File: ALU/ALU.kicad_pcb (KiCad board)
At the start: 2 copper layers, 115 x 57 mm, 33 parts, among them J1 Conn_01x06_Pin, J2 Conn_01x08_Pin, J3 Conn_01x08_Pin, J4 Conn_01x10_Pin, U1 SN74F86N, U2 SN74F86N, U3 SN74HCT245N, U4 CD74HCT283E, U5 CD74HCT283E, U8 Dual D FF

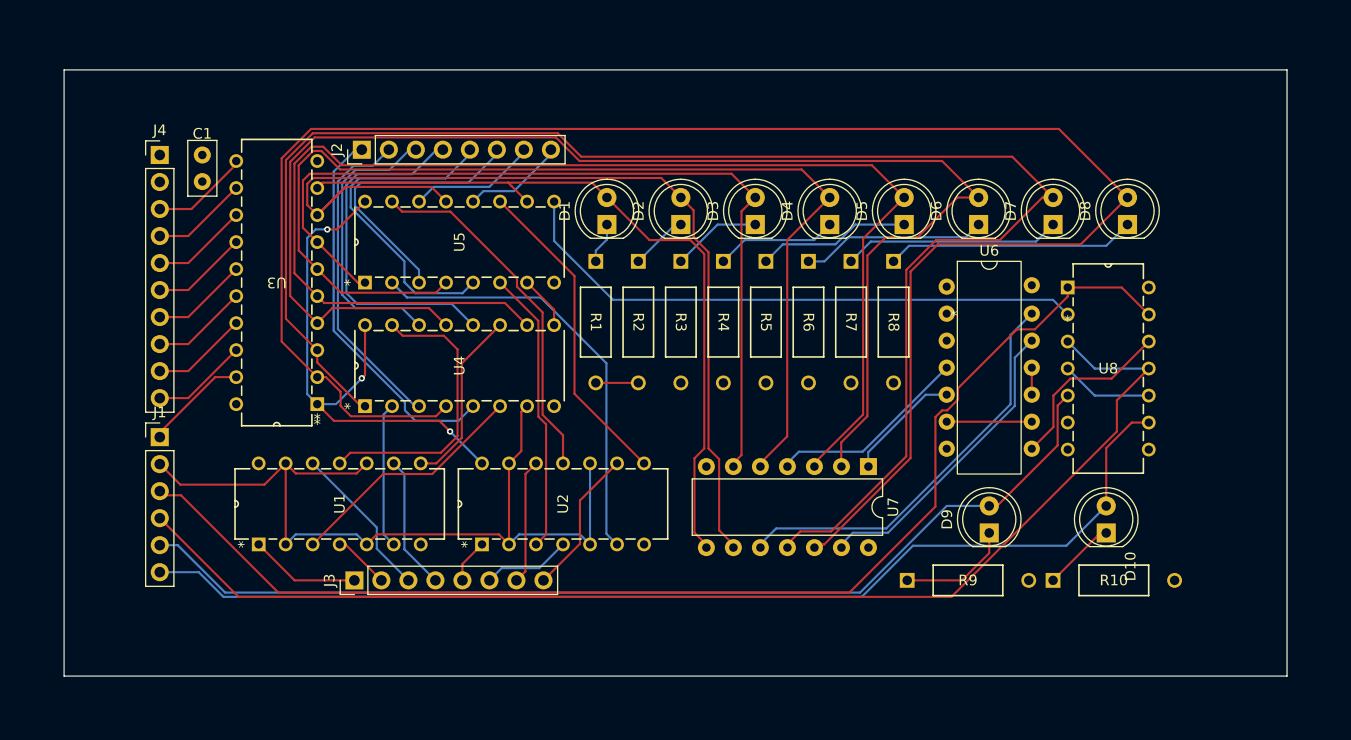
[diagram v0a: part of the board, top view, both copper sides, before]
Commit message: ALU layout complete
ALU layout complete
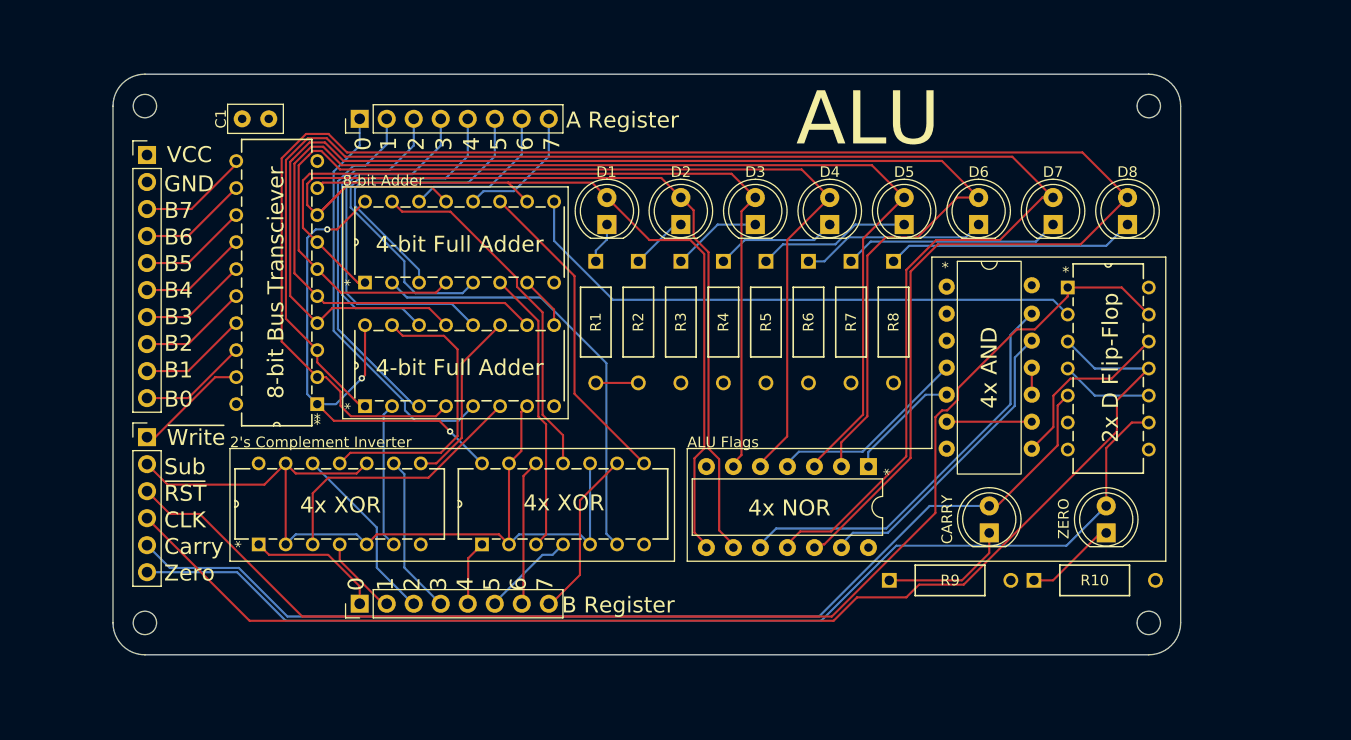
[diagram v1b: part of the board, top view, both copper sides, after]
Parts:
- added REF**: MountingHole_2.2mm_M2, MountingHole:MountingHole_2.2mm_M2, F.Cu at (78.6, 134.0)
- added REF**: MountingHole_2.2mm_M2, MountingHole:MountingHole_2.2mm_M2, F.Cu at (173.0, 134.0)
- added REF**: MountingHole_2.2mm_M2, MountingHole:MountingHole_2.2mm_M2, F.Cu at (78.6, 85.4)
- added REF**: MountingHole_2.2mm_M2, MountingHole:MountingHole_2.2mm_M2, F.Cu at (173.0, 85.4)
- moved C1 5.06 mm to (87.8, 86.6), turned to 0 degrees
- moved J2 2.91 mm to (98.8, 86.6)
- moved J3 2.26 mm to (98.8, 132.2)
- moved R10 1.80 mm to (162.2, 130.0)
- moved R9 1.69 mm to (148.6, 130.0)
- moved J1 1.20 mm to (78.8, 116.5)
- moved J4 1.20 mm to (78.8, 90.0)
- renumbered D9 to CARRY, D10 to ZERO
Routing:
- net /~{RST}: track 115.9 -> 119.4 mm
- net /CLK: track 115.3 -> 118.4 mm
- net /CARRY: track 97.1 -> 100.2 mm
- net /ZERO: track 103.9 -> 107.0 mm
- net /A6: track 12.0 -> 14.9 mm
- net /A7: track 9.59 -> 12.4 mm
- net /A5: track 26.5 -> 29.3 mm
- net /A4: track 31.3 -> 34.1 mm
- net /XOR0: track 23.0 -> 25.8 mm
- net /A3: track 33.8 -> 36.2 mm
- net /A2: track 27.1 -> 29.6 mm
- net /A0: track 36.1 -> 38.6 mm
- net /B2: track 14.7 -> 17.2 mm
- net /B3: track 12.6 -> 15.0 mm
- net /A1: track 30.5 -> 32.9 mm
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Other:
- board size 115 x 57 mm -> 100.4 x 54.6 mm
- board text added: "0"
- board text added: "1"
- board text added: "2"
- board text added: "2's Complement Inverter"
- board text added: "2x D Flip-Flop"
- board text added: "3"
- board text added: "4"
- board text added: "4-bit Full Adder"
- board text added: "4x AND"
- board text added: "4x NOR"
- board text added: "4x XOR"
- board text added: "5"
- board text added: "6"
- board text added: "7"
- board text added: "8-bit Adder"
- board text added: "8-bit Bus Transciever"
- board text added: "A Register"
- board text added: "ALU"
- board text added: "ALU Flags"
- board text added: "B Register"
- board text added: "B0"
- board text added: "B1"
- board text added: "B2"
- board text added: "B3"
- board text added: "B4"
- board text added: "B5"
- board text added: "B6"
- board text added: "B7"
- board text added: "CLK"
- board text added: "Carry"
- board text added: "GND"
- board text added: "Sub"
- board text added: "VCC"
- board text added: "Zero"
- board text added: "~{RST}"
- board text added: "~{Write}"
